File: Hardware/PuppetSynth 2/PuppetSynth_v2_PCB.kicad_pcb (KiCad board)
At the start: 2 copper layers, 165.8 x 155.2 mm, 43 parts, among them J10 PINHD_1x6_Female, J11 JST_03, J12 JST_03, J13 JST_05, J14 JST_05, J15 JST_05, J16 JST_03, J19 PINHD_1x6_Female, J20 JST_03, J24 JST_03, J25 JST_03, J26 JST_03, J3 JST_03, J5 JST_05, J8 PINHD_1x6_Female, J9 PINHD_1x6_Female

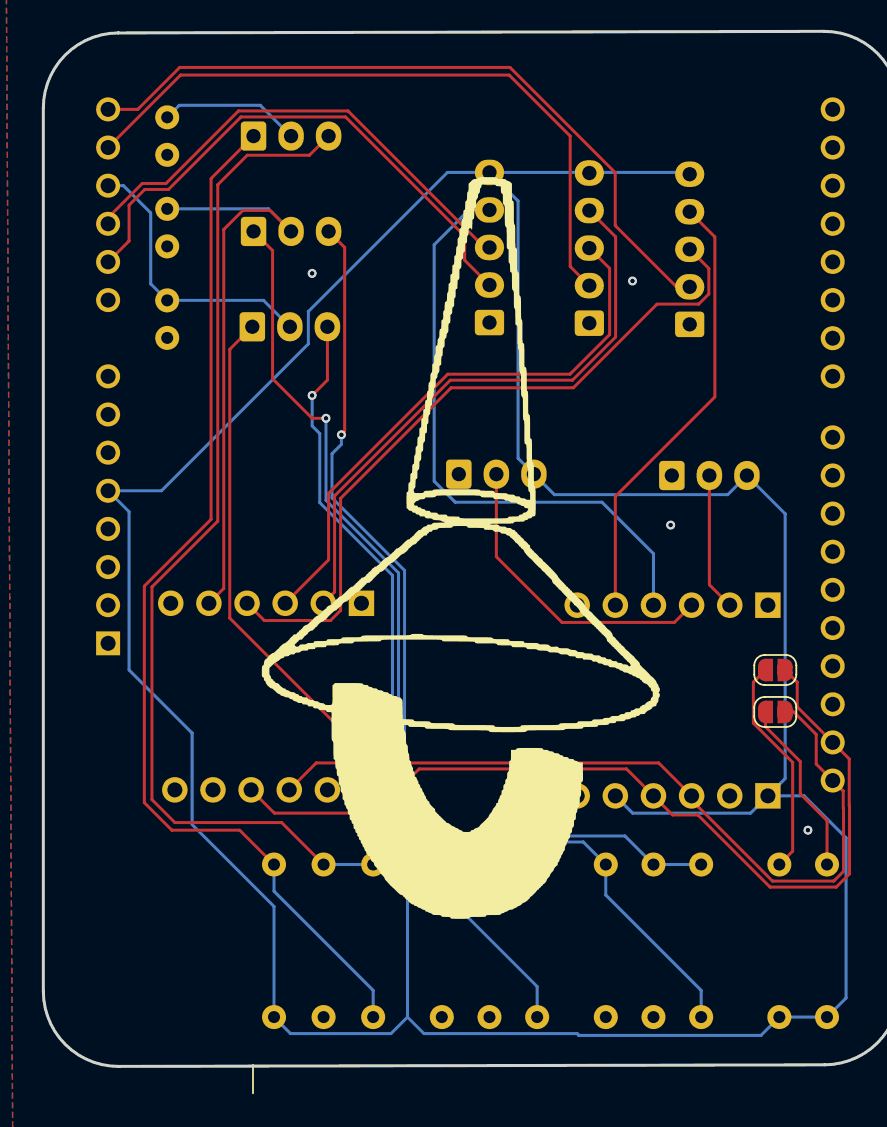
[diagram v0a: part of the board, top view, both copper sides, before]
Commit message: minor fixes
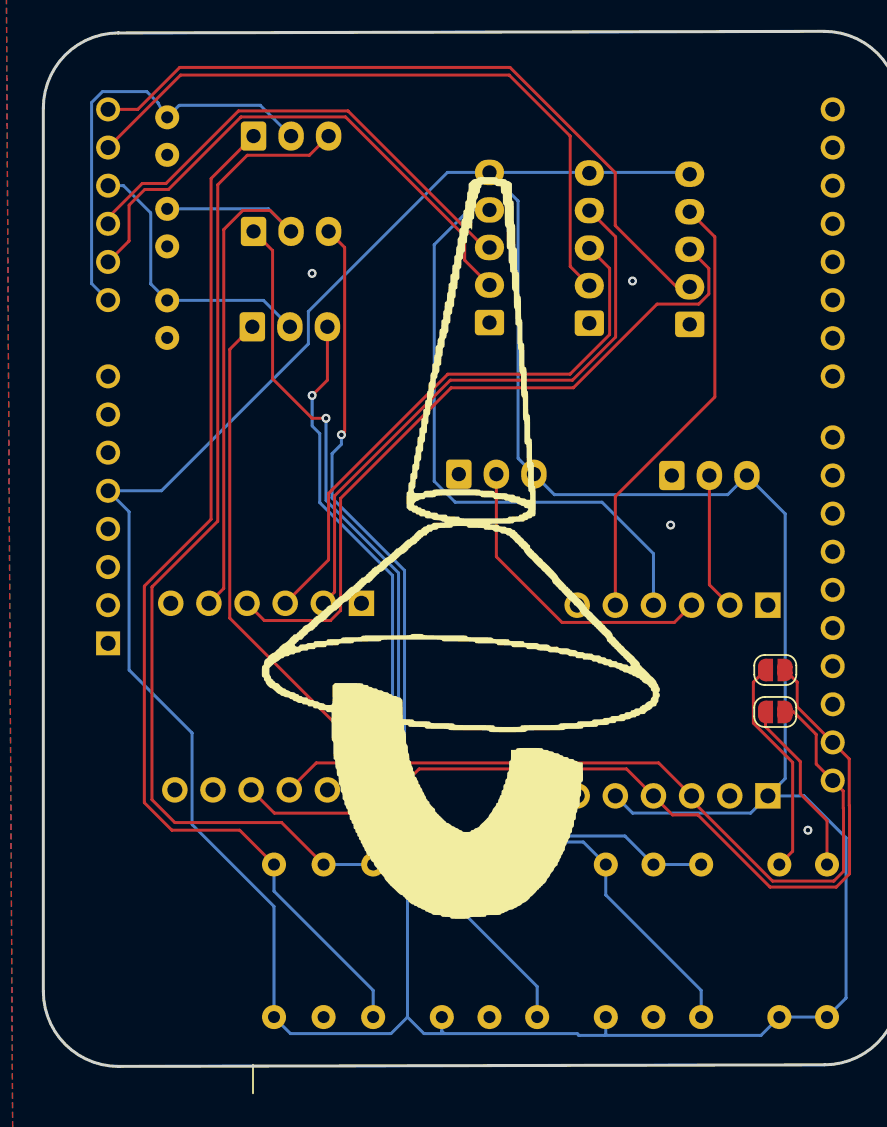
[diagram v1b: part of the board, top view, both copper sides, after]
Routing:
- net Toggle_1: track 0.00 -> 18.7 mm
- net +5V: track 267.3 -> 269.8 mm
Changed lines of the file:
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@@
 		(fp_arc
 			(start -1.4 -0.300001)
-			(mid -1.194974 -0.794976)
+			(mid -1.194975 -0.794976)
 			(end -0.699999 -0.999999)
 			(stroke
@@
 		(fp_arc
 			(start 0.7 -1.000001)
-			(mid 1.194973 -0.794975)
+			(mid 1.194975 -0.794975)
 			(end 1.399998 -0.3)
 			(stroke
@@
 		(fp_arc
 			(start -1.4 -0.300001)
-			(mid -1.194974 -0.794976)
+			(mid -1.194975 -0.794976)
 			(end -0.699999 -0.999999)
 			(stroke
@@
 		(fp_arc
 			(start 0.7 -1.000001)
-			(mid 1.194973 -0.794975)
+			(mid 1.194975 -0.794975)
 			(end 1.399998 -0.3)
 			(stroke
@@
 		)
 	)
+	(gr_line
+		(start 190.5 40.894)
+		(end 190.754 41.402)
+		(stroke
+			(width 0.2)
+			(type default)
+		)
+		(layer "B.Cu")
+	)
 	(gr_poly
 		(pts
@@
 	)
 	(segment
-		(start 208.201065 102.869122)
-		(end 218.409177 102.869121)
-		(width 0.2)
-		(layer "B.Cu")
-		(net 33)
-	)
-	(segment
 		(start 136.983 124.466648)
 		(end 136.983 124.451001)
@@
 	)
 	(segment
-		(start 218.531061 102.991006)
-		(end 230.644178 102.991001)
-		(width 0.2)
-		(layer "B.Cu")
-		(net 33)
-	)
-	(segment
 		(start 204.30706 87.545117)
 		(end 207.10106 90.339121)
@@
 	)
 	(segment
+		(start 218.531061 102.991006)
+		(end 220.218 102.991005)
+		(width 0.2)
+		(layer "B.Cu")
+		(net 33)
+	)
+	(segment
 		(start 206.001062 102.869118)
 		(end 207.101062 101.769122)
@@
 	)
 	(segment
+		(start 209.387062 102.706184)
+		(end 209.55 102.869122)
+		(width 0.2)
+		(layer "B.Cu")
+		(net 33)
+	)
+	(segment
 		(start 214.467059 64.557651)
 		(end 214.46706 47.420114)
@@
 	)
 	(segment
+		(start 209.55 102.869122)
+		(end 218.409177 102.869121)
+		(width 0.2)
+		(layer "B.Cu")
+		(net 33)
+	)
+	(segment
 		(start 207.101062 101.769122)
 		(end 208.201065 102.869122)
@@
 	)
 	(segment
+		(start 220.218 102.991005)
+		(end 230.644178 102.991001)
+		(width 0.2)
+		(layer "B.Cu")
+		(net 33)
+	)
+	(segment
 		(start 187.162063 66.717118)
 		(end 190.718062 66.71712)
@@
 	)
 	(segment
+		(start 220.309062 102.899943)
+		(end 220.218 102.991005)
+		(width 0.2)
+		(layer "B.Cu")
+		(net 33)
+	)
+	(segment
 		(start 231.866062 101.769118)
 		(end 232.501057 101.769118)
@@
 	)
 	(segment
+		(start 209.387062 101.769119)
+		(end 209.387062 102.706184)
+		(width 0.2)
+		(layer "B.Cu")
+		(net 33)
+	)
+	(segment
 		(start 232.254064 85.887121)
 		(end 232.254063 68.248119)
@@
 	)
 	(segment
+		(start 208.201065 102.869122)
+		(end 209.55 102.869122)
+		(width 0.2)
+		(layer "B.Cu")
+		(net 33)
+	)
+	(segment
 		(start 192.757059 82.85312)
 		(end 188.559064 78.655119)
@@
 	)
 	(segment
+		(start 220.309062 101.76911)
+		(end 220.309062 102.899943)
+		(width 0.2)
+		(layer "B.Cu")
+		(net 33)
+	)
+	(segment
 		(start 220.944064 87.03712)
 		(end 222.094064 88.187121)
@@
 	)
 	(segment
+		(start 186.791541 40.132)
+		(end 189.738 40.132)
+		(width 0.2)
+		(layer "B.Cu")
+		(net 48)
+	)
+	(segment
+		(start 189.738 40.132)
+		(end 190.5 40.894)
+		(width 0.2)
+		(layer "B.Cu")
+		(net 48)
+	)
+	(segment
+		(start 187.162061 54.017117)
+		(end 186.062061 52.917117)
+		(width 0.2)
+		(layer "B.Cu")
+		(net 48)
+	)
+	(segment
+		(start 186.062061 40.86148)
+		(end 186.791541 40.132)
+		(width 0.2)
+		(layer "B.Cu")
+		(net 48)
+	)
+	(segment
+		(start 186.062061 52.917117)
+		(end 186.062061 40.86148)
+		(width 0.2)
+		(layer "B.Cu")
+		(net 48)
+	)
+	(segment
